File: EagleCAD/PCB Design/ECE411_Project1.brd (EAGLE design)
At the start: 160 x 100 mm, 39 parts, among them J1 0473460001_USBMICRO, U1 ATS160SM-1, U2 MIC29310-5.0WU, U3 NCP5501DT50RKG, U4 DCJACK_2.1MM_PTH

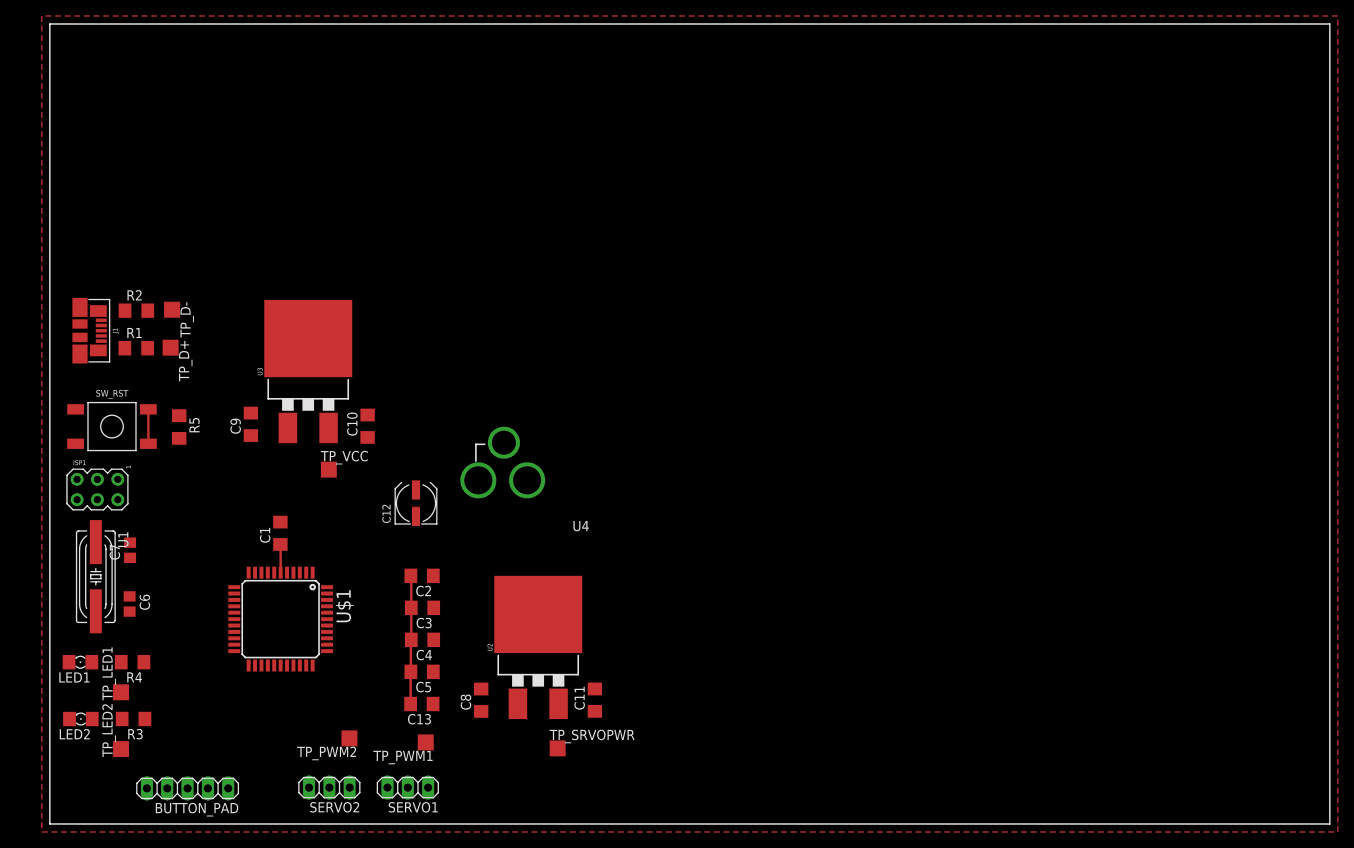
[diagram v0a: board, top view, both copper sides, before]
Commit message: In progress - almost finished layout
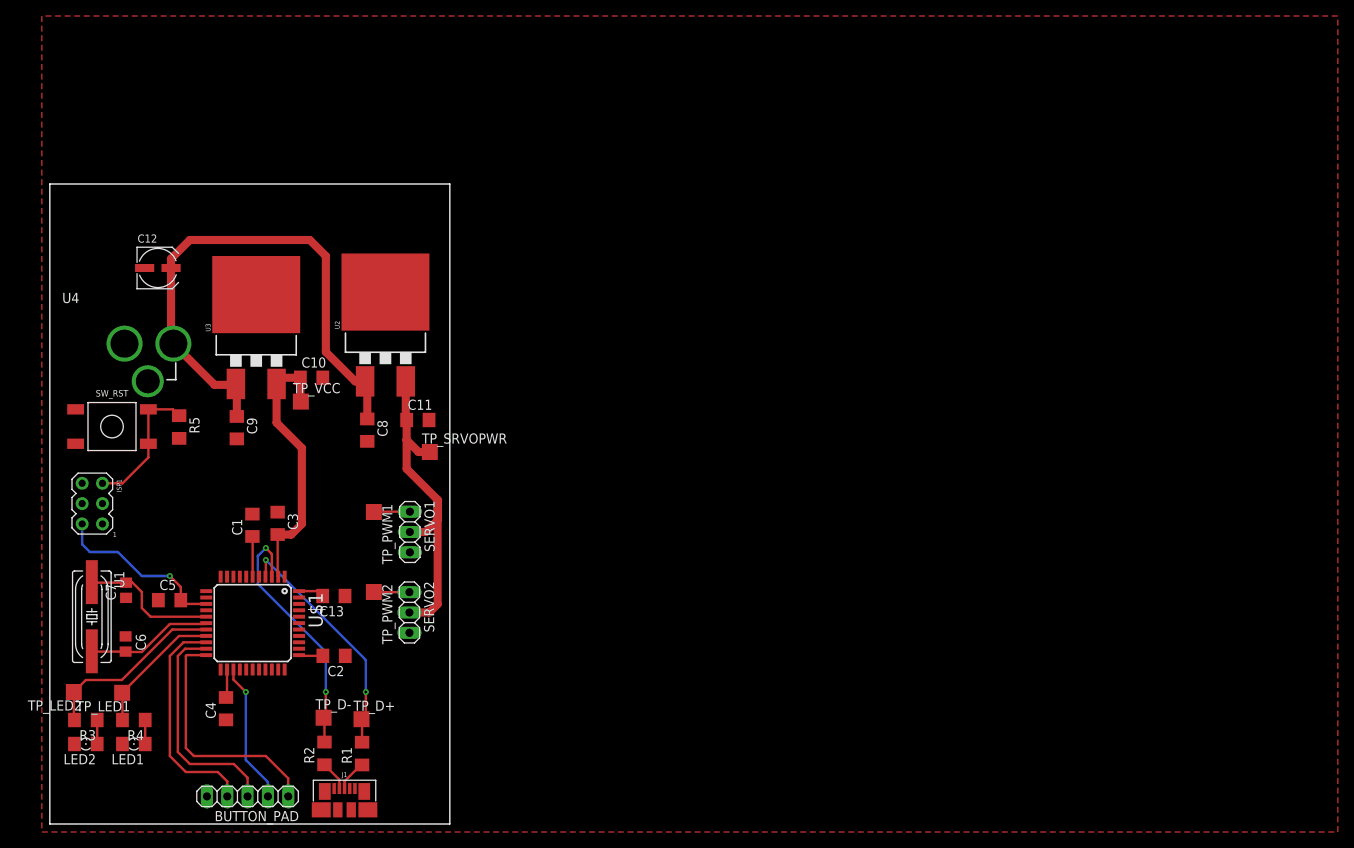
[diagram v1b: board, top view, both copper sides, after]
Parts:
- moved J1 68.4 mm to (36.8, 1.77), turned to 90 degrees
- moved U4 68.1 mm to (1.54, 60.0), turned to 270 degrees
- moved R2 60.1 mm to (34.3, 8.82), turned to 90 degrees
- moved R1 58.0 mm to (39.0, 8.80), turned to 90 degrees
- moved TP_D- 54.4 mm to (34.2, 13.3), turned to 0 degrees
- moved TP_D+ 52.2 mm to (39.0, 13.1), turned to 0 degrees
- moved U2 44.6 mm to (42.0, 62.4)
- moved C12 43.7 mm to (13.5, 69.5), turned to 0 degrees
- moved C11 41.4 mm to (46.0, 50.5), turned to 0 degrees
- moved TP_SRVOPWR 40.3 mm to (47.5, 46.5)
- moved C8 36.6 mm to (39.7, 49.2), turned to 270 degrees
- moved C5 32.8 mm to (15.0, 28.0), turned to 0 degrees
- moved SERVO1 32.0 mm to (45.0, 36.5), turned to 270 degrees
- moved TP_PWM1 29.5 mm to (40.5, 39.0), turned to 270 degrees
- moved C4 26.0 mm to (22.0, 14.4), turned to 90 degrees
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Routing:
- net UNREG_PWR: track 0.00 -> 70.6 mm
- net VCC: track 16.9 -> 65.9 mm, vias 0 -> 1
- net SERVO_PWR: track 0.00 -> 44.1 mm
- net D-MCU: track 0.00 -> 32.5 mm, vias 0 -> 2
- net N$13: track 0.00 -> 30.7 mm
- net D+MCU: track 0.00 -> 30.4 mm, vias 0 -> 2
- net N$11: track 0.00 -> 28.3 mm
- net N$7: track 0.00 -> 28.1 mm
- net N$6: track 0.00 -> 23.3 mm
- net N$12: track 0.00 -> 17.6 mm, vias 0 -> 1
- net XTAL2: track 0.00 -> 17.3 mm
- net N$8: track 0.00 -> 16.9 mm
- net XTAL1: track 0.00 -> 15.8 mm
- net /RST: track 4.30 -> 17.3 mm
- net PWM1: track 0.00 -> 4.52 mm
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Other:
- board size 160 x 100 mm -> 50 x 80 mm
